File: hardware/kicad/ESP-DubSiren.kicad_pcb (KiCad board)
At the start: 2 copper layers, 15.6 x 2.1 mm, 68 parts, among them J1 USB4085-GF-A, J2 NRJ4HF, SW1 MX2A-11NW, SW2 MX2A-11NW, SW3 MX2A-11NW, SW4 MX2A-11NW, SW5 RESET, SW6 BOOT, SW7 PEC11R-4120F-S0018, U1 ESP32-S3-WROOM-1U-N16R8, U2 MPM3612GLQ-33-Z, U3 74HC4051D, U4 USBLC6-2SC6, U5 Adafruit 5393, U6 Adafruit 6250, U7 TPS22918DBVR

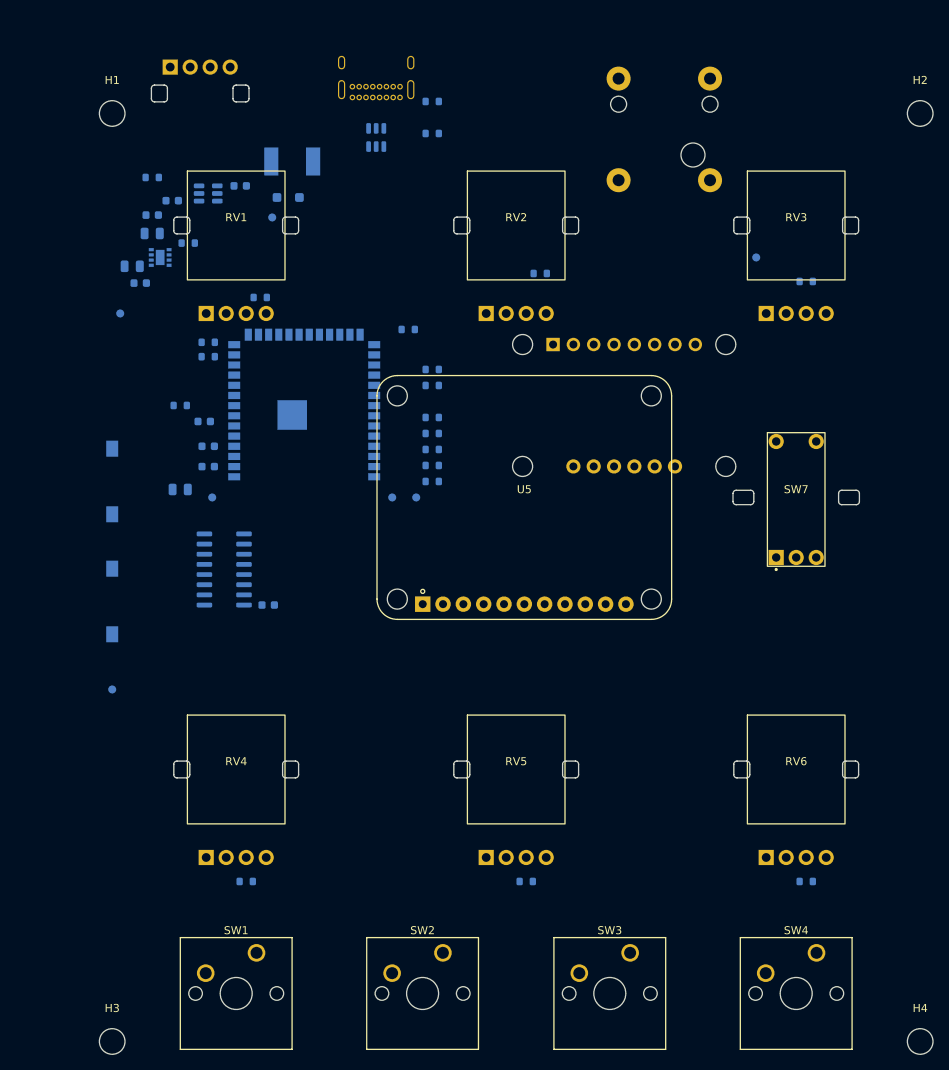
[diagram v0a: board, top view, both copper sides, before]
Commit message: Review electrical design and propose standalone PCB layout (#34, #35)
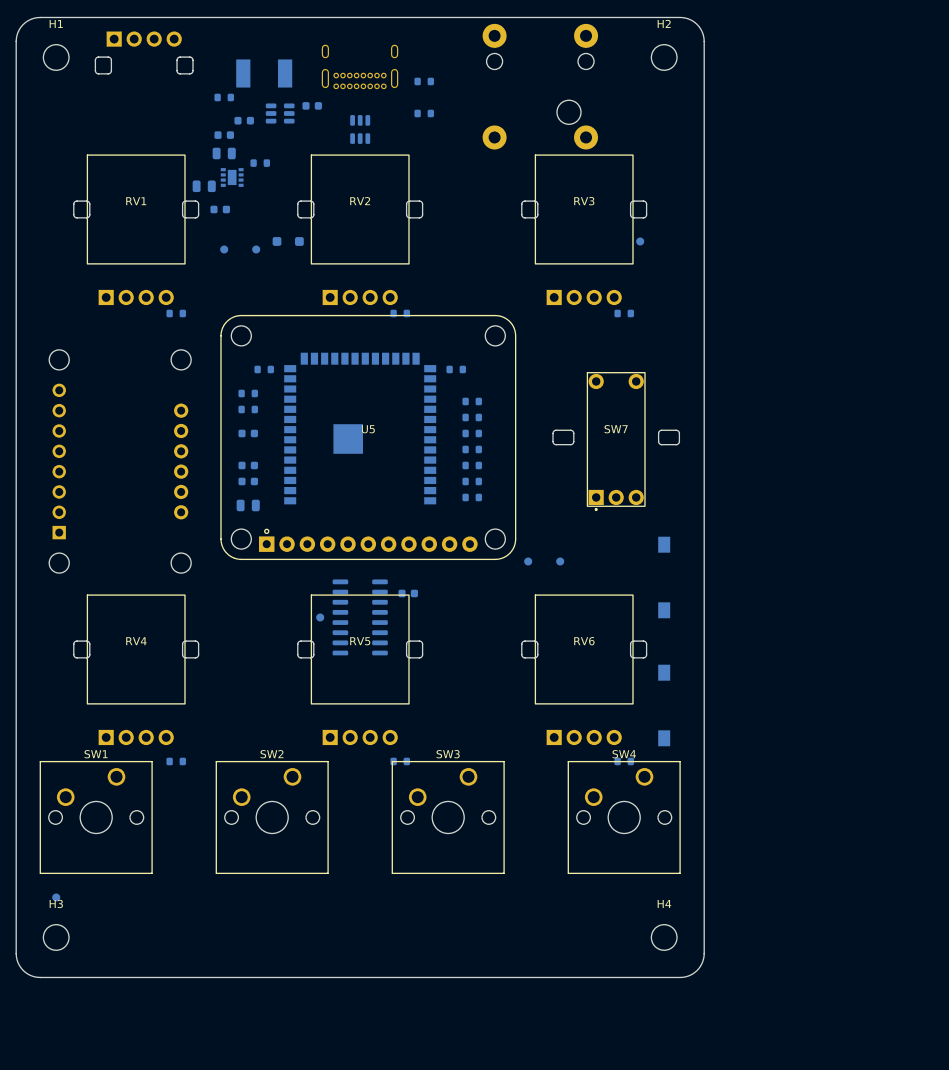
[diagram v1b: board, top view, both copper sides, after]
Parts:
- moved SW6 70.2 mm to (81.0, 86.0)
- moved SW5 70.0 mm to (81.0, 70.0)
- moved U6 63.4 mm to (13.0, 55.5), turned to 90 degrees
- moved H4 34.5 mm to (81.0, 115.0)
- moved H2 32.8 mm to (81.0, 5.00)
- moved SW4 30.8 mm to (78.5, 94.9)
- moved RV6 30.5 mm to (71.0, 79.0)
- moved SW3 29.9 mm to (56.5, 94.9)
- moved SW2 28.9 mm to (34.5, 94.9)
- moved SW1 28.1 mm to (12.5, 94.9)
- moved R13 27.2 mm to (76.0, 93.0)
- moved TP3 26.9 mm to (5.00, 110.0)
- moved RV3 26.6 mm to (71.0, 24.0)
- moved RV5 24.6 mm to (43.0, 79.0)
- moved SW7 23.7 mm to (75.0, 52.5)
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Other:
- board size 15.6 x 2.1 mm -> 86 x 120 mm
- board text added: "86 x 120 mm / R3 / M3 D3.2"
- board text added: "H1-H4: KEEP FREE 8x8 mm BOTH SIDES"
- board text added: "KEYCAP 20x20: UNVERIFIED"
